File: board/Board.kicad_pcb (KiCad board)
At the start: 2 copper layers, 50.8 x 56.3 mm, 59 parts, among them J1 GS3, J10 CONN_01X03, J11 CONN_01X03, J12 GS3, J13 GS3, J14 CONN_01X02, J15 CONN_01X03, J16 GS2, J17 CONN_01X01, J2 CONN_02X04, J3 CONN_01X03, J4 CONN_01X03, J5 CONN_01X03, J6 CONN_01X03, J7 CONN_01X03, J8 CONN_01X03, J9 CONN_01X03, SW1 SW_Push, U1 STM32F410RBTx, U2 SN74LVC1G04, U3 LF33ABDT-TR, U4 ICM-20689, U5 MAG3110, U6 MS5637, Y1 25 MHz

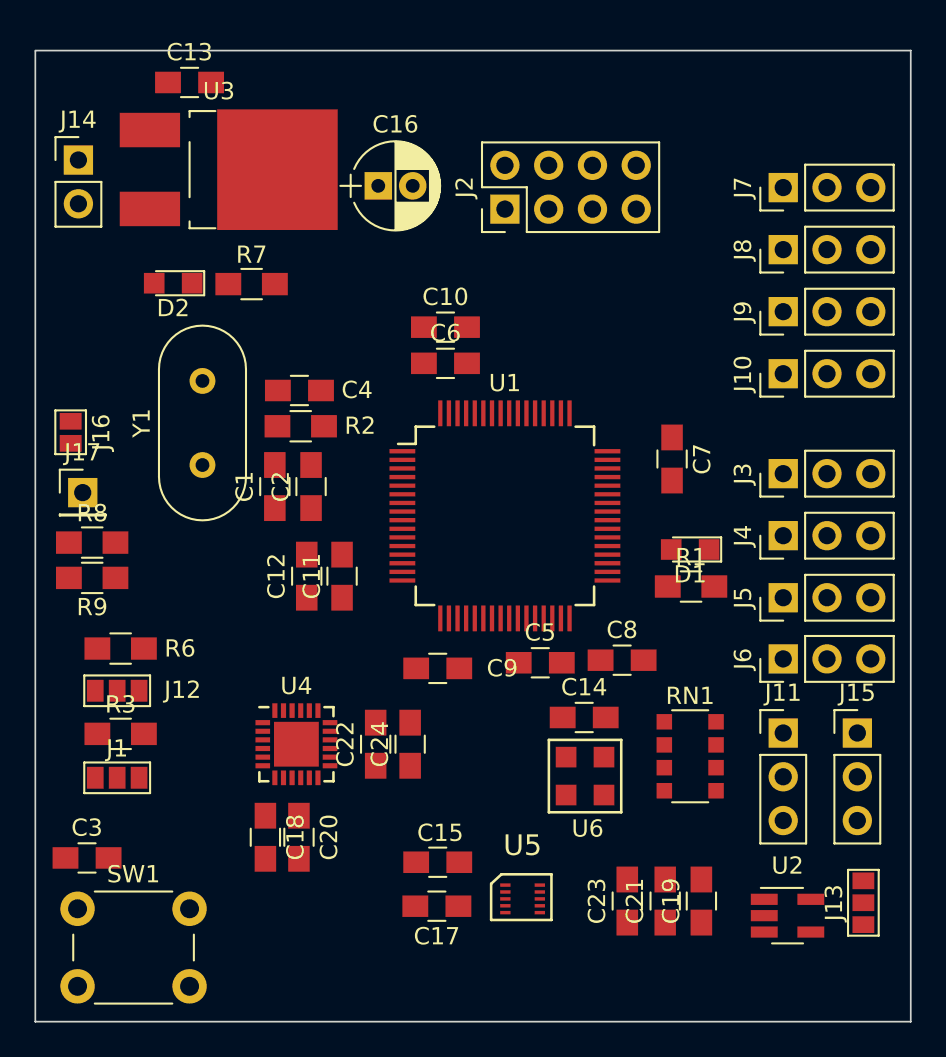
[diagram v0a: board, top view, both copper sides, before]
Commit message: 50x50mm
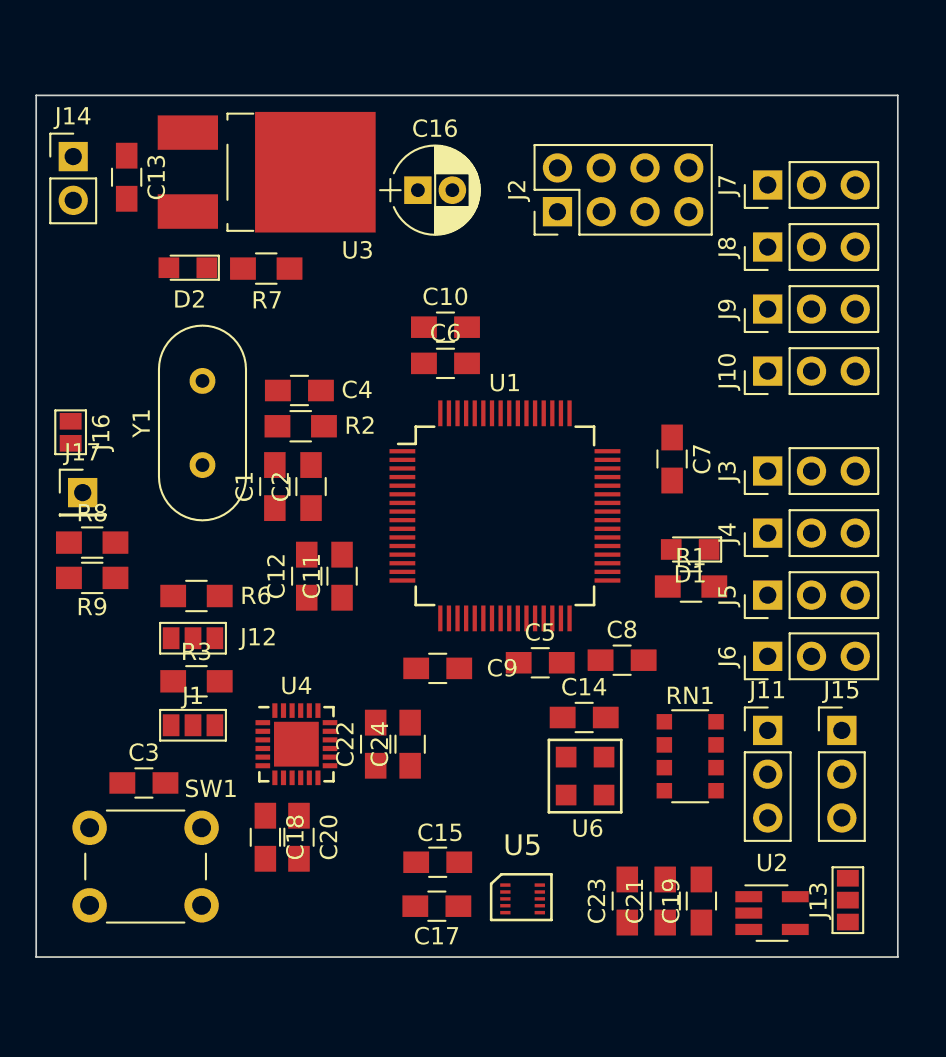
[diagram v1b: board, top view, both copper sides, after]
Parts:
- moved C13 6.60 mm to (108.5, 75.8), turned to 270 degrees
- moved C3 5.46 mm to (109.5, 111.0)
- moved J12 5.35 mm to (112.4, 102.6)
- moved J1 5.35 mm to (112.4, 107.7)
- moved R3 5.35 mm to (112.6, 105.1)
- moved R6 5.35 mm to (112.6, 100.2)
- moved SW1 4.75 mm to (106.4, 113.6)
- moved J2 3.05 mm to (133.6, 77.8)
- moved C16 2.31 mm to (125.5, 76.6)
- moved U3 2.21 mm to (115.8, 75.5)
- moved D2 1.24 mm to (112.1, 81.1)
- moved R7 1.24 mm to (116.7, 81.2)
- moved J10 0.91 mm to (145.8, 87.1)
- moved J13 0.91 mm to (150.4, 117.8)
- moved J4 0.91 mm to (145.8, 96.5)
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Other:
- board size 50.8 x 56.3 mm -> 50 x 50 mm
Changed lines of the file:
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@@
     (links 151)
     (no_connects 151)
-    (area 100.716667 67.625 212.358334 166.235)
+    (area 103.199999 68.449999 154.100001 124.900001)
     (thickness 1.6)
     (drawings 4)
@@
   )
   (module Capacitors_SMD:C_0805_HandSoldering (layer F.Cu)
-    (at 106.25 115.35)
+    (at 109.55 111)
     (descr "Capacitor SMD 0805, hand soldering")
     (tags "capacitor 0805")
@@
   )
   (module Capacitors_SMD:C_0805_HandSoldering (layer F.Cu)
-    (at 112.2 70.35)
+    (at 108.55 75.85 270)
     (descr "Capacitor SMD 0805, hand soldering")
     (tags "capacitor 0805")
     (attr smd)
-    (fp_text reference C13 (at 0 -1.75) (layer F.SilkS)
-      (effects (font (size 1 1) (thickness 0.15)))
-    )
-    (fp_text value 0.1uF (at 0 1.75) (layer F.Fab)
-      (effects (font (size 1 1) (thickness 0.15)))
-    )
-    (fp_text user %R (at 0 -1.75) (layer F.Fab)
+    (fp_text reference C13 (at 0 -1.75 270) (layer F.SilkS)
+      (effects (font (size 1 1) (thickness 0.15)))
+    )
+    (fp_text value 0.1uF (at 0 1.75 270) (layer F.Fab)
+      (effects (font (size 1 1) (thickness 0.15)))
+    )
+    (fp_text user %R (at 0 -1.75 270) (layer F.Fab)
       (effects (font (size 1 1) (thickness 0.15)))
     )
@@
     (fp_line (start 2.25 0.87) (end 2.25 -0.88) (layer F.CrtYd) (width 0.05))
     (fp_line (start 2.25 0.87) (end -2.25 0.87) (layer F.CrtYd) (width 0.05))
-    (pad 1 smd rect (at -1.25 0) (size 1.5 1.25) (layers F.Cu F.Paste F.Mask)
+    (pad 1 smd rect (at -1.25 0 270) (size 1.5 1.25) (layers F.Cu F.Paste F.Mask)
       (net 7 +BATT))
-    (pad 2 smd rect (at 1.25 0) (size 1.5 1.25) (layers F.Cu F.Paste F.Mask)
+    (pad 2 smd rect (at 1.25 0 270) (size 1.5 1.25) (layers F.Cu F.Paste F.Mask)
       (net 1 GND))
     (model Capacitors_SMD.3dshapes/C_0805.wrl
@@
   )
   (module Capacitors_ThroughHole:CP_Radial_D5.0mm_P2.00mm (layer F.Cu)
-    (at 123.15 76.35)
+    (at 125.45 76.6)
     (descr "CP, Radial series, Radial, pin pitch=2.00mm, , diameter=5mm, Electrolytic Capacitor")
     (tags "CP Radial series Radial pin pitch 2.00mm  diameter 5mm Electrolytic Capacitor")
@@
   )
   (module LEDs:LED_0805 (layer F.Cu)
-    (at 111.25 82 180)
+    (at 112.1 81.1 180)
     (descr "LED 0805 smd package")
     (tags "LED led 0805 SMD smd SMT smt smdled SMDLED smtled SMTLED")
     (attr smd)
-    (fp_text reference D2 (at 0 -1.45 180) (layer F.SilkS)
+    (fp_text reference D2 (at -0.1 -1.85 180) (layer F.SilkS)
       (effects (font (size 1 1) (thickness 0.15)))
     )
@@
   )
   (module Connect:GS3 (layer F.Cu)
-    (at 108 110.7 270)
+    (at 112.4 107.65 270)
     (descr "3-pin solder bridge")
     (tags "solder bridge")
@@
   )
   (module Pin_Headers:Pin_Header_Straight_2x04_Pitch2.54mm (layer F.Cu)
-    (at 130.5 77.7 90)
+    (at 133.55 77.85 90)
     (descr "Through hole straight pin header, 2x04, 2.54mm pitch, double rows")
     (tags "Through hole pin header THT 2x04 2.54mm double row")
@@
   )
   (module Pin_Headers:Pin_Header_Straight_1x03_Pitch2.54mm (layer F.Cu)
-    (at 146.65 93.05 90)
+    (at 145.75 92.9 90)
     (descr "Through hole straight pin header, 1x03, 2.54mm pitch, single row")
     (tags "Through hole pin header THT 1x03 2.54mm single row")
@@
   )
   (module Pin_Headers:Pin_Header_Straight_1x03_Pitch2.54mm (layer F.Cu)
-    (at 146.65 96.65 90)
+    (at 145.75 96.5 90)
     (descr "Through hole straight pin header, 1x03, 2.54mm pitch, single row")
     (tags "Through hole pin header THT 1x03 2.54mm single row")
@@
   )
   (module Pin_Headers:Pin_Header_Straight_1x03_Pitch2.54mm (layer F.Cu)
-    (at 146.65 100.25 90)
+    (at 145.75 100.1 90)
     (descr "Through hole straight pin header, 1x03, 2.54mm pitch, single row")
     (tags "Through hole pin header THT 1x03 2.54mm single row")
@@
   )
   (module Pin_Headers:Pin_Header_Straight_1x03_Pitch2.54mm (layer F.Cu)
-    (at 146.65 103.8 90)
+    (at 145.75 103.65 90)
     (descr "Through hole straight pin header, 1x03, 2.54mm pitch, single row")
     (tags "Through hole pin header THT 1x03 2.54mm single row")
@@
   )
   (module Pin_Headers:Pin_Header_Straight_1x03_Pitch2.54mm (layer F.Cu)
-    (at 146.65 76.45 90)
+    (at 145.75 76.3 90)
     (descr "Through hole straight pin header, 1x03, 2.54mm pitch, single row")
     (tags "Through hole pin header THT 1x03 2.54mm single row")
@@
   )
   (module Pin_Headers:Pin_Header_Straight_1x03_Pitch2.54mm (layer F.Cu)
-    (at 146.65 80.05 90)
+    (at 145.75 79.9 90)
     (descr "Through hole straight pin header, 1x03, 2.54mm pitch, single row")
     (tags "Through hole pin header THT 1x03 2.54mm single row")
@@
   )
   (module Pin_Headers:Pin_Header_Straight_1x03_Pitch2.54mm (layer F.Cu)
-    (at 146.65 83.65 90)
+    (at 145.75 83.5 90)
     (descr "Through hole straight pin header, 1x03, 2.54mm pitch, single row")
     (tags "Through hole pin header THT 1x03 2.54mm single row")
@@
   )
   (module Pin_Headers:Pin_Header_Straight_1x03_Pitch2.54mm (layer F.Cu)
-    (at 146.65 87.25 90)
+    (at 145.75 87.1 90)
     (descr "Through hole straight pin header, 1x03, 2.54mm pitch, single row")
     (tags "Through hole pin header THT 1x03 2.54mm single row")
@@
   )
   (module Pin_Headers:Pin_Header_Straight_1x03_Pitch2.54mm (layer F.Cu)
-    (at 146.65 108.1)
+    (at 145.75 107.95)
     (descr "Through hole straight pin header, 1x03, 2.54mm pitch, single row")
     (tags "Through hole pin header THT 1x03 2.54mm single row")
@@
   )
   (module Connect:GS3 (layer F.Cu)
-    (at 108 105.65 270)
+    (at 112.4 102.6 270)
     (descr "3-pin solder bridge")
     (tags "solder bridge")
@@
   )
   (module Connect:GS3 (layer F.Cu)
-    (at 151.3 117.95)
+    (at 150.4 117.8)
     (descr "3-pin solder bridge")
     (tags "solder bridge")
@@
   )
   (module Pin_Headers:Pin_Header_Straight_1x02_Pitch2.54mm (layer F.Cu)
-    (at 105.75 74.85)
+    (at 105.45 74.65)
     (descr "Through hole straight pin header, 1x02, 2.54mm pitch, single row")
     (tags "Through hole pin header THT 1x02 2.54mm single row")
@@
   )
   (module Pin_Headers:Pin_Header_Straight_1x03_Pitch2.54mm (layer F.Cu)
-    (at 150.95 108.1)
+    (at 150.05 107.95)
     (descr "Through hole straight pin header, 1x03, 2.54mm pitch, single row")
     (tags "Through hole pin header THT 1x03 2.54mm single row")
@@
   )
   (module Resistors_SMD:R_0805_HandSoldering (layer F.Cu)
-    (at 108.2 108.15)
+    (at 112.6 105.1)
     (descr "Resistor SMD 0805, hand soldering")
     (tags "resistor 0805")
@@
   )
   (module Resistors_SMD:R_0805_HandSoldering (layer F.Cu)
-    (at 108.2 103.2 180)
+    (at 112.6 100.15 180)
     (descr "Resistor SMD 0805, hand soldering")
     (tags "resistor 0805")
@@
   )
   (module Resistors_SMD:R_0805_HandSoldering (layer F.Cu)
-    (at 115.8 82.05)
+    (at 116.65 81.15)
     (descr "Resistor SMD 0805, hand soldering")
     (tags "resistor 0805")
     (attr smd)
-    (fp_text reference R7 (at 0 -1.7) (layer F.SilkS)
+    (fp_text reference R7 (at 0.05 1.85) (layer F.SilkS)
       (effects (font (size 1 1) (thickness 0.15)))
     )
@@
   )
   (module Buttons_Switches_ThroughHole:SW_PUSH_6mm (layer F.Cu)
-    (at 105.7 118.3)
+    (at 106.4 113.6)
     (descr https://www.omron.com/ecb/products/pdf/en-b3f.pdf)
     (tags "tact sw push 6mm")
-    (fp_text reference SW1 (at 3.25 -2) (layer F.SilkS)
+    (fp_text reference SW1 (at 7.05 -2.25) (layer F.SilkS)
       (effects (font (size 1 1) (thickness 0.15)))
     )
@@
   )
   (module TO_SOT_Packages_SMD:SOT-23-5_HandSoldering (layer F.Cu)
-    (at 146.9 118.7)
+    (at 146 118.55)
     (descr "5-pin SOT23 package")
     (tags "SOT-23-5 hand-soldering")
@@
   )
   (module TO_SOT_Packages_SMD:TO-252-2Lead (layer F.Cu)
-    (at 113.6 75.4)
+    (at 115.8 75.55)
     (descr TO-252-2Lead)
     (tags "TO-252 2Lead")
     (attr smd)
-    (fp_text reference U3 (at 0.3 -4.54) (layer F.SilkS)
+    (fp_text reference U3 (at 6.15 4.55) (layer F.SilkS)
       (effects (font (size 1 1) (thickness 0.15)))
     )
@@
     )
   )
-  (gr_line (start 154.05 68.5) (end 103.25 68.5) (angle 90) (layer Edge.Cuts) (width 0.1))
-  (gr_line (start 154.05 124.85) (end 154.05 68.5) (angle 90) (layer Edge.Cuts) (width 0.1))
-  (gr_line (start 103.25 124.85) (end 154.05 124.85) (angle 90) (layer Edge.Cuts) (width 0.1))
-  (gr_line (start 103.25 68.55) (end 103.25 124.85) (angle 90) (layer Edge.Cuts) (width 0.1))
+  (gr_line (start 153.3 121.1) (end 103.3 121.1) (angle 90) (layer Edge.Cuts) (width 0.1))
+  (gr_line (start 153.3 71.1) (end 153.3 121.1) (angle 90) (layer Edge.Cuts) (width 0.1))
+  (gr_line (start 153.3 71.1) (end 103.3 71.1) (angle 90) (layer Edge.Cuts) (width 0.1))
+  (gr_line (start 103.3 71.1) (end 103.3 121.1) (angle 90) (layer Edge.Cuts) (width 0.1))
 )
